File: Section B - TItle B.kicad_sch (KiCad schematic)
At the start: 1 part

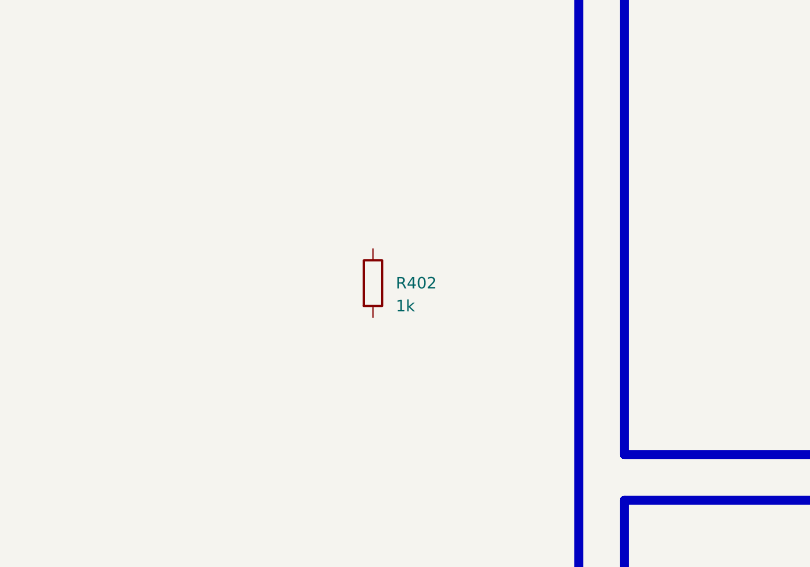
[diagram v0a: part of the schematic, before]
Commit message: Revert "section-a: also tweak section B"
This reverts commit 97cee964c54efe81b466f277d38d322d4de4fe3f.
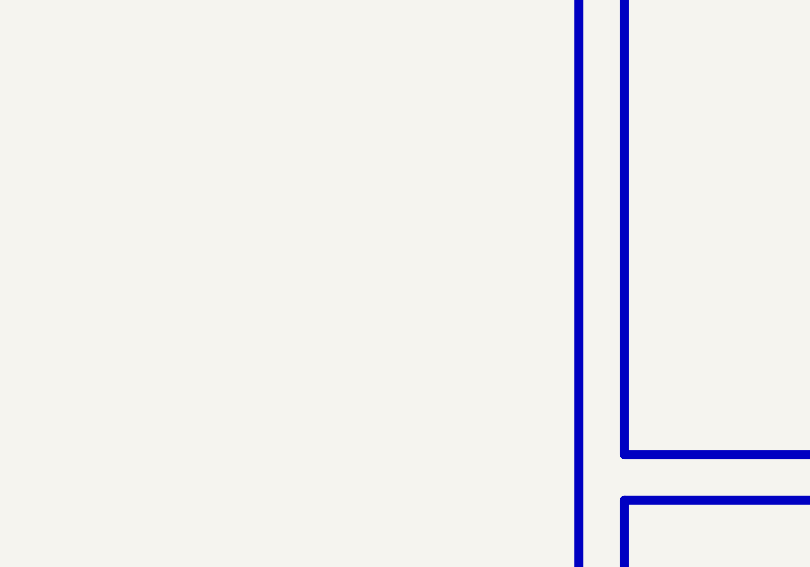
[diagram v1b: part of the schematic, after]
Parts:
- removed R402: 1k, Resistor_SMD:R_0603_1608Metric, symbol Device:R
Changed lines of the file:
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@@
-		)
-	)
-	(symbol
-		(lib_id "Device:R")
-		(at 111.76 101.6 0)
-		(unit 1)
-		(exclude_from_sim no)
-		(in_bom yes)
-		(on_board yes)
-		(dnp no)
-		(property "Reference" "R402"
-			(at 114.30000000000001 101.6 0)
-			(effects (font (size 1.27 1.27)) (justify left))
-		)
-		(property "Value" "1k"
-			(at 114.30000000000001 104.14 0)
-			(effects (font (size 1.27 1.27)) (justify left))
-		)
-		(property "Footprint" "Resistor_SMD:R_0603_1608Metric"
-			(at 111.76 101.6 0)
-			(effects (font (size 1.27 1.27)) (hide yes))
-		)
-		(property "Datasheet" "~"
-			(at 111.76 101.6 0)
-			(effects (font (size 1.27 1.27)) (hide yes))
-		)
-		(pin "1")
-		(pin "2")
-		(instances
-			(project "ci_dummy"
-				(path "/f9e05184-c88b-4a88-ae9c-ab2bdb32be7c/c5103ceb-5325-4a84-a025-9638a412984e/e744f3ce-03a6-44a6-8792-1447ef232b9a"
-					(reference "R402")
-					(unit 1)
-				)
-			)
 		)
 	)

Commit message: section-a: also tweak section B
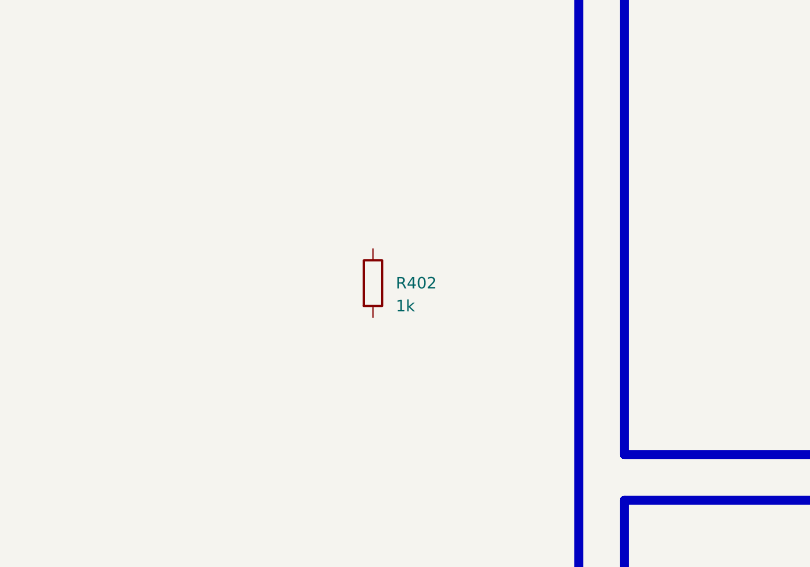
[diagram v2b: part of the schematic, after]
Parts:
- added R402: 1k, Resistor_SMD:R_0603_1608Metric, symbol Device:R
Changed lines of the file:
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@@
+		)
+	)
+	(symbol
+		(lib_id "Device:R")
+		(at 111.76 101.6 0)
+		(unit 1)
+		(exclude_from_sim no)
+		(in_bom yes)
+		(on_board yes)
+		(dnp no)
+		(property "Reference" "R402"
+			(at 114.30000000000001 101.6 0)
+			(effects (font (size 1.27 1.27)) (justify left))
+		)
+		(property "Value" "1k"
+			(at 114.30000000000001 104.14 0)
+			(effects (font (size 1.27 1.27)) (justify left))
+		)
+		(property "Footprint" "Resistor_SMD:R_0603_1608Metric"
+			(at 111.76 101.6 0)
+			(effects (font (size 1.27 1.27)) (hide yes))
+		)
+		(property "Datasheet" "~"
+			(at 111.76 101.6 0)
+			(effects (font (size 1.27 1.27)) (hide yes))
+		)
+		(pin "1")
+		(pin "2")
+		(instances
+			(project "ci_dummy"
+				(path "/f9e05184-c88b-4a88-ae9c-ab2bdb32be7c/c5103ceb-5325-4a84-a025-9638a412984e/e744f3ce-03a6-44a6-8792-1447ef232b9a"
+					(reference "R402")
+					(unit 1)
+				)
+			)
 		)
 	)
